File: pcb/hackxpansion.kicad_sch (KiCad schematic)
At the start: 0 parts

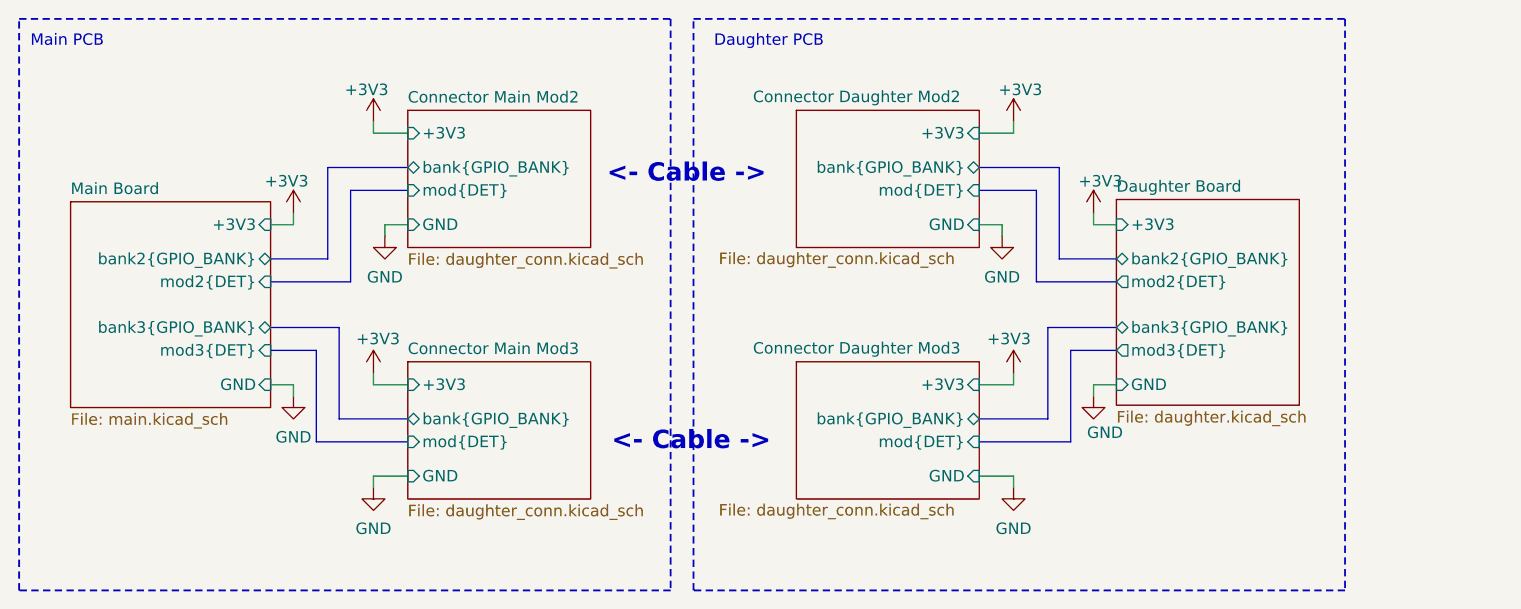
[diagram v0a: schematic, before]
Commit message: moved stuff around
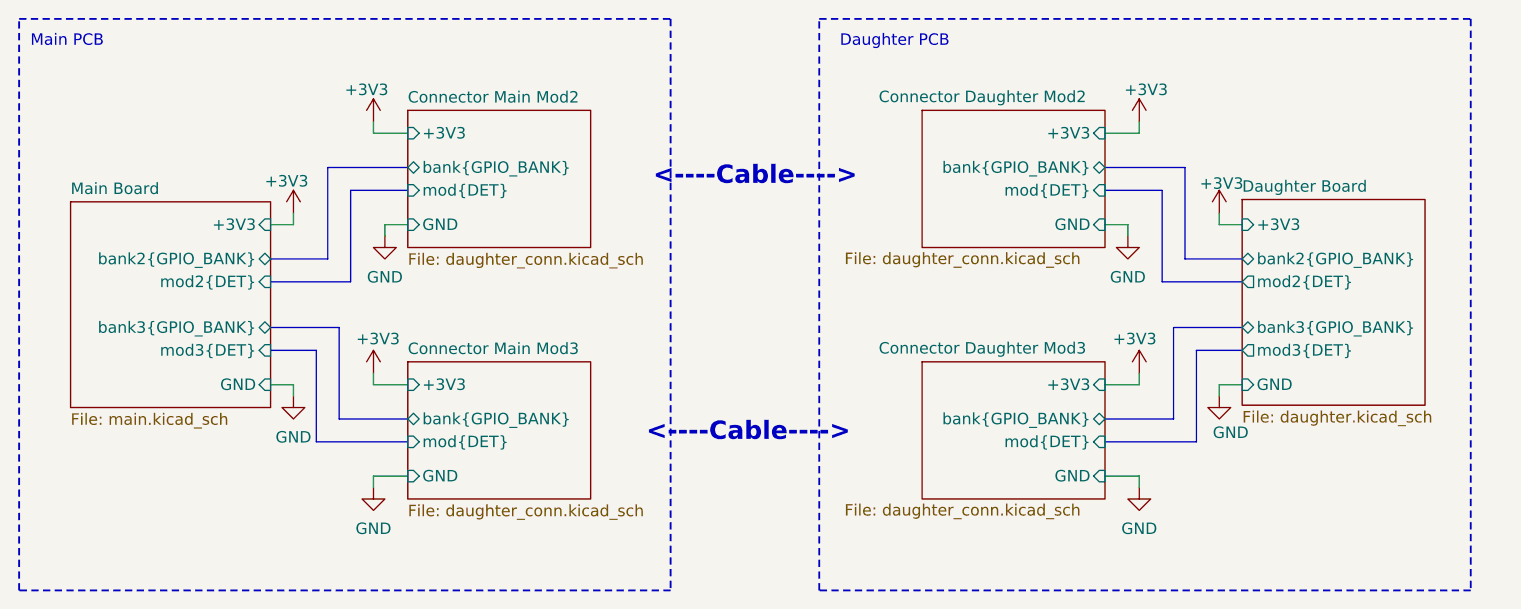
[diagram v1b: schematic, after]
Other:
- note added: "<----Cable---->"
- note removed: "<- Cable ->"
